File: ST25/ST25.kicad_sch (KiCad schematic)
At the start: 41 parts, among them J1 Conn_01x13, J2 Conn_01x13, J3 Conn_01x13, J4 Conn_01x08, J5 Conn_01x08, SW1 [1], SW10 [*], SW11 [0], SW12 [#], SW13 [1], SW14 [2], SW15 [3], SW16 [4], SW17 [5], SW18 [6], SW19 [7], SW2 [2], SW20 [8], SW21 [9], SW22 [*], SW23 [0], SW24 [#], SW3 [3], SW4 [4], SW5 [5], SW6 [6], SW7 [7], SW8 [8], SW9 [9], U1 HEF4094B, U2 HEF4094B

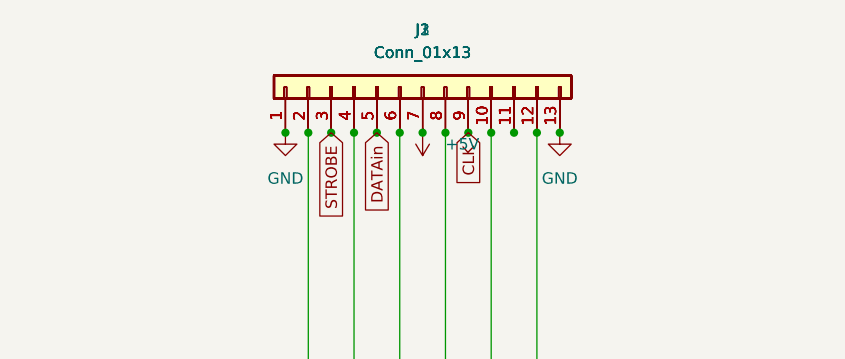
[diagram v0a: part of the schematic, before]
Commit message: ffc
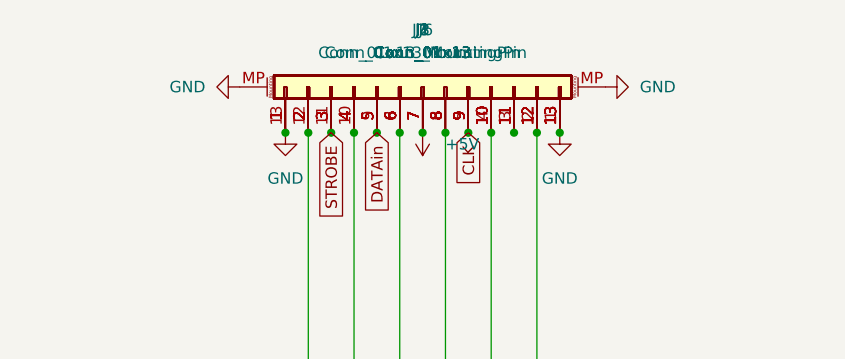
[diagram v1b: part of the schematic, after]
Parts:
- added J6: Conn_01x13_MountingPin, Connector_FFC-FPC:TE_1-84952-3_1x13-1MP_P1.0mm_Horizontal, symbol Connector_Generic_MountingPin:Conn_01x13_MountingPin
- added J7: Conn_01x13_MountingPin, Connector_FFC-FPC:TE_1-84953-3_1x13-1MP_P1.0mm_Horizontal, symbol Connector_Generic_MountingPin:Conn_01x13_MountingPin
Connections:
- net +5V: now also J6.7 (Pin_7), J7.7 (Pin_7)
- net CLK: now also J6.9 (Pin_9), J7.5 (Pin_5)
- net DATAin: now also J6.5 (Pin_5), J7.9 (Pin_9)
- net GND: now also J6.1 (Pin_1), J6.13 (Pin_13), J6.MP (MountPin), J7.1 (Pin_1), J7.13 (Pin_13), J7.MP (MountPin)
- net STROBE: now also J6.3 (Pin_3), J7.11 (Pin_11)
- net at J1.4 (Pin_4), J2.4 (Pin_4), J3.4 (Pin_4)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: now also J6.4 (Pin_4), J7.10 (Pin_10)
- net at J1.2 (Pin_2), J2.2 (Pin_2), J3.2 (Pin_2)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: now also J6.2 (Pin_2), J7.12 (Pin_12)
- net at J1.10 (Pin_10), J2.10 (Pin_10), J3.10 (Pin_10)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: now also J6.10 (Pin_10), J7.4 (Pin_4)
- net at J1.6 (Pin_6), J2.6 (Pin_6), J3.6 (Pin_6)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: now also J6.6 (Pin_6), J7.8 (Pin_8)
- net at J1.12 (Pin_12), J2.12 (Pin_12), J3.12 (Pin_12)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: now also J6.12 (Pin_12), J7.2 (Pin_2)
- net at J1.8 (Pin_8), J2.8 (Pin_8), J3.8 (Pin_8)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: now also J6.8 (Pin_8), J7.6 (Pin_6)
- net at J1.11 (Pin_11), J2.11 (Pin_11), J3.11 (Pin_11): now also J6.11 (Pin_11), J7.3 (Pin_3)

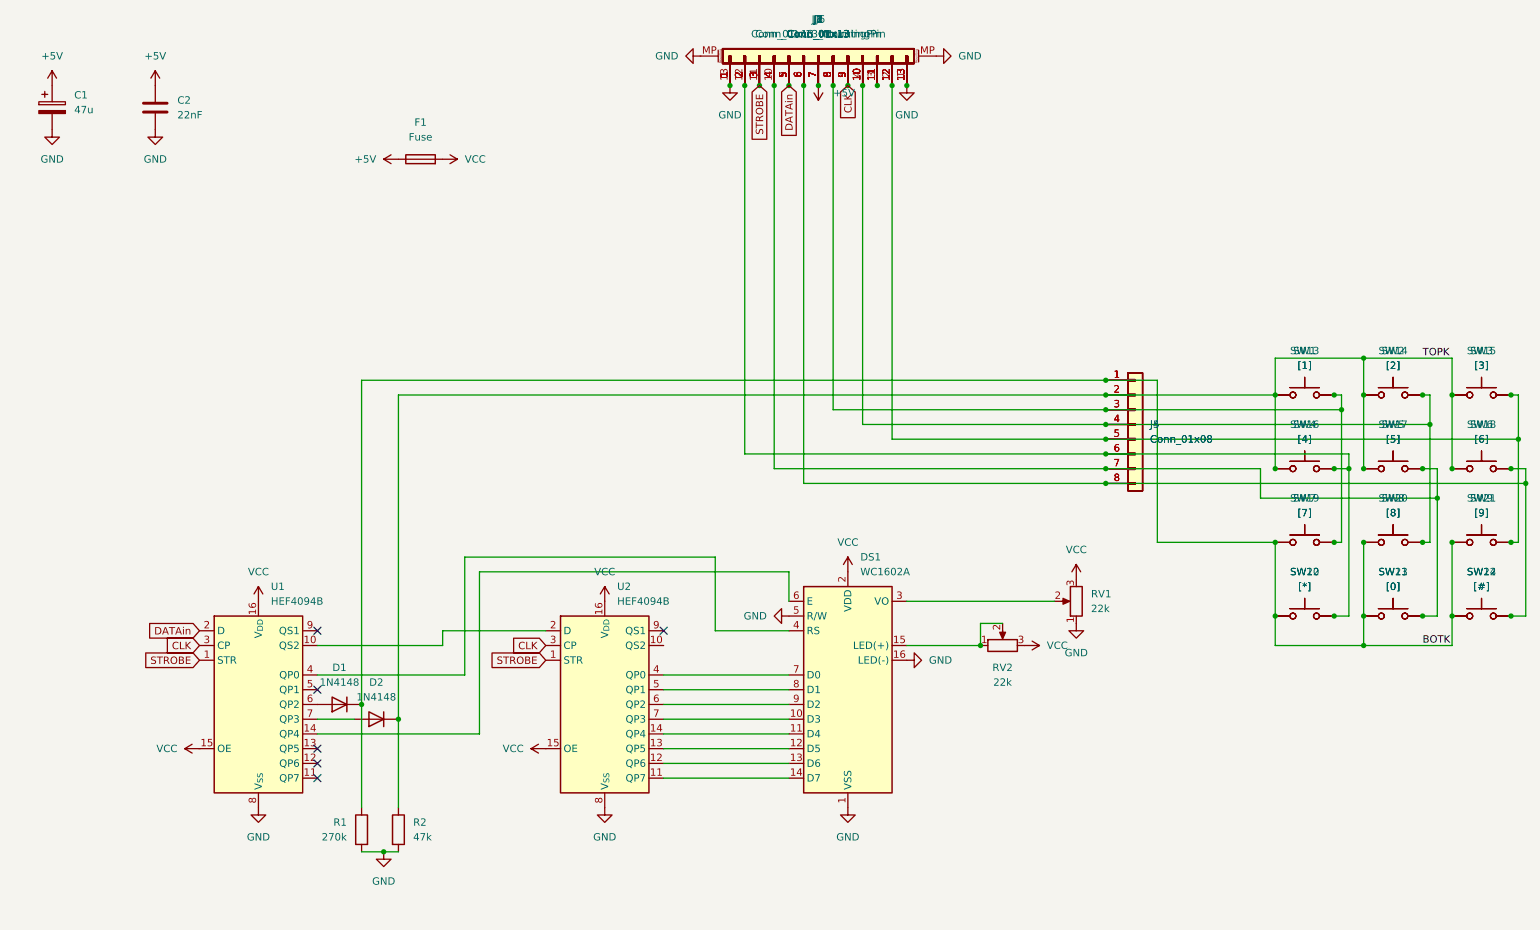
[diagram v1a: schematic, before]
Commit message: led und ffc
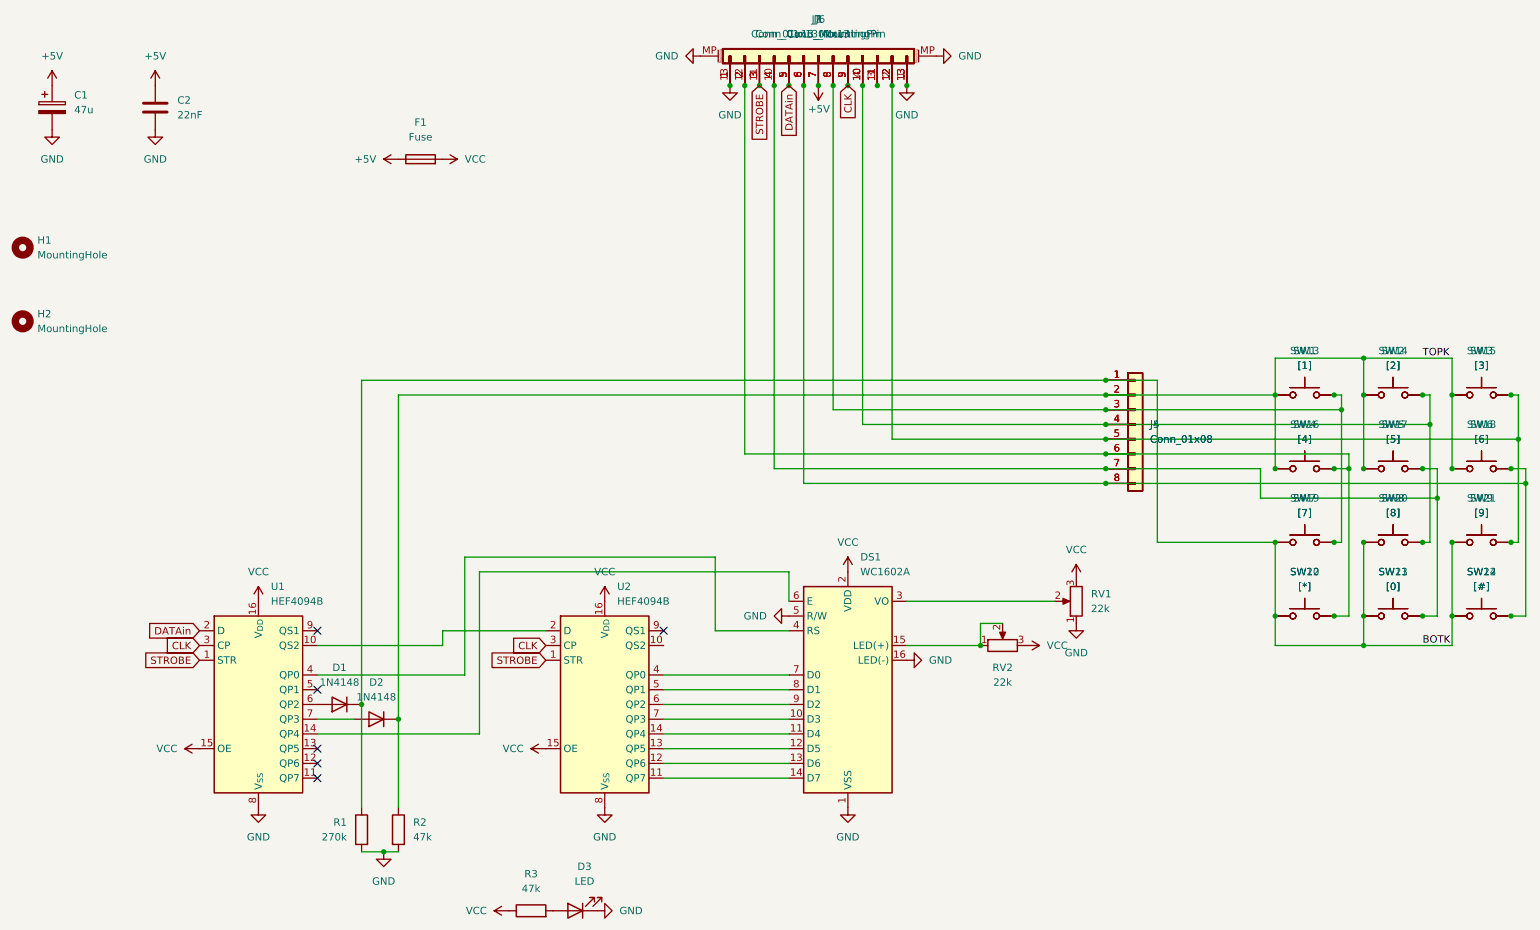
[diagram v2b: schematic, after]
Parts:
- removed J2, J3: Conn_01x13, Connector_PinHeader_2.54mm:PinHeader_1x13_P2.54mm_Vertical, symbol Connector_Generic:Conn_01x13
- added D3: LED, LED_SMD:LED_0603_1608Metric, symbol Device:LED
- added H1, H2: MountingHole, MountingHole:MountingHole_3mm, symbol Mechanical:MountingHole
- added R3: 47k, Resistor_SMD:R_0603_1608Metric, symbol Device:R
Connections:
- net GND: now also D3.1 (K)
- net VCC: now also R3.1
- new net: D3.2 (A), R3.2

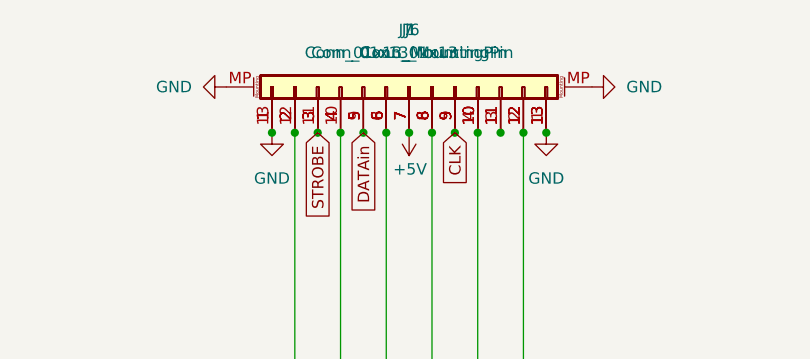
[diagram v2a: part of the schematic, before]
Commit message: loecher dann doch
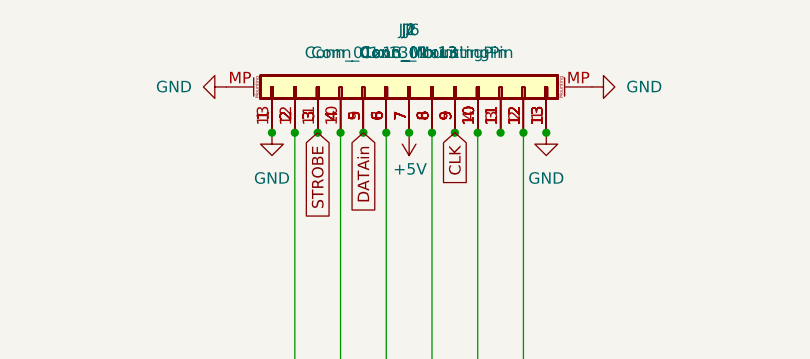
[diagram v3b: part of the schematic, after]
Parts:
- added J2: Conn_01x13, Connector_PinHeader_2.54mm:PinHeader_1x13_P2.54mm_Vertical, symbol Connector_Generic:Conn_01x13
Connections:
- net +5V: now also J2.7 (Pin_7)
- net CLK: now also J2.9 (Pin_9)
- net DATAin: now also J2.5 (Pin_5)
- net GND: now also J2.1 (Pin_1), J2.13 (Pin_13)
- net STROBE: now also J2.3 (Pin_3)
- net at J1.4 (Pin_4), J4.7 (Pin_7), J5.7 (Pin_7)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: now also J2.4 (Pin_4)
- net at J1.2 (Pin_2), J4.6 (Pin_6), J5.6 (Pin_6)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: now also J2.2 (Pin_2)
- net at J1.10 (Pin_10), J4.4 (Pin_4), J5.4 (Pin_4)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: now also J2.10 (Pin_10)
- net at J1.6 (Pin_6), J4.8 (Pin_8), J5.8 (Pin_8)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: now also J2.6 (Pin_6)
- net at J1.11 (Pin_11), J6.11 (Pin_11), J7.3 (Pin_3): now also J2.11 (Pin_11)
- net at J1.12 (Pin_12), J4.5 (Pin_5), J5.5 (Pin_5)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: now also J2.12 (Pin_12)
- net at J1.8 (Pin_8), J4.3 (Pin_3), J5.3 (Pin_3)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: now also J2.8 (Pin_8)
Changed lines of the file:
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@@
+		(dnp no)
+		(fields_autoplaced yes)
+		(property "Reference" "J2"
+			(at 162.56 24.13 90)
+			(effects
+				(font
+					(size 1.27 1.27)
+				)
+			)
+		)
+		(property "Value" "Conn_01x13"
+			(at 162.56 26.67 90)
+			(effects
+				(font
+					(size 1.27 1.27)
+				)
+			)
+		)
+		(property "Footprint" "Connector_PinHeader_2.54mm:PinHeader_1x13_P2.54mm_Vertical"
+			(at 162.56 30.48 0)
+			(effects
+				(font
+					(size 1.27 1.27)
+				)
+				(hide yes)
+			)
+		)
+		(property "Datasheet" "~"
+			(at 162.56 30.48 0)
+			(effects
+				(font
+					(size 1.27 1.27)
+				)
+				(hide yes)
+			)
+		)
+		(property "Description" "Generic connector, single row, 01x13, script generated (kicad-library-utils/schlib/autogen/connector/)"
+			(at 162.56 30.48 0)
+			(effects
+				(font
+					(size 1.27 1.27)
+				)
+				(hide yes)
+			)
+		)
+		(pin "8"
+		)
+		(pin "1"
+		)
+		(pin "4"
+		)
+		(pin "3"
+		)
+		(pin "2"
+		)
+		(pin "13"
+		)
+		(pin "5"
+		)
+		(pin "6"
+		)
+		(pin "9"
+		)
+		(pin "11"
+		)
+		(pin "12"
+		)
+		(pin "7"
+		)
+		(pin "10"
+		)
+		(instances
+			(project ""
+				(path "/37c1adda-ac5c-405e-8496-b0b1b030189c"
+					(reference "J2")
+					(unit 1)
+				)
+			)
+		)
+	)
+	(symbol
+		(lib_id "Connector_Generic:Conn_01x13")
+		(at 162.56 30.48 90)
+		(unit 1)
+		(exclude_from_sim no)
+		(in_bom yes)
+		(on_board yes)
 		(dnp no)
 		(fields_autoplaced yes)
